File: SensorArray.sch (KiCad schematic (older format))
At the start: 13 parts

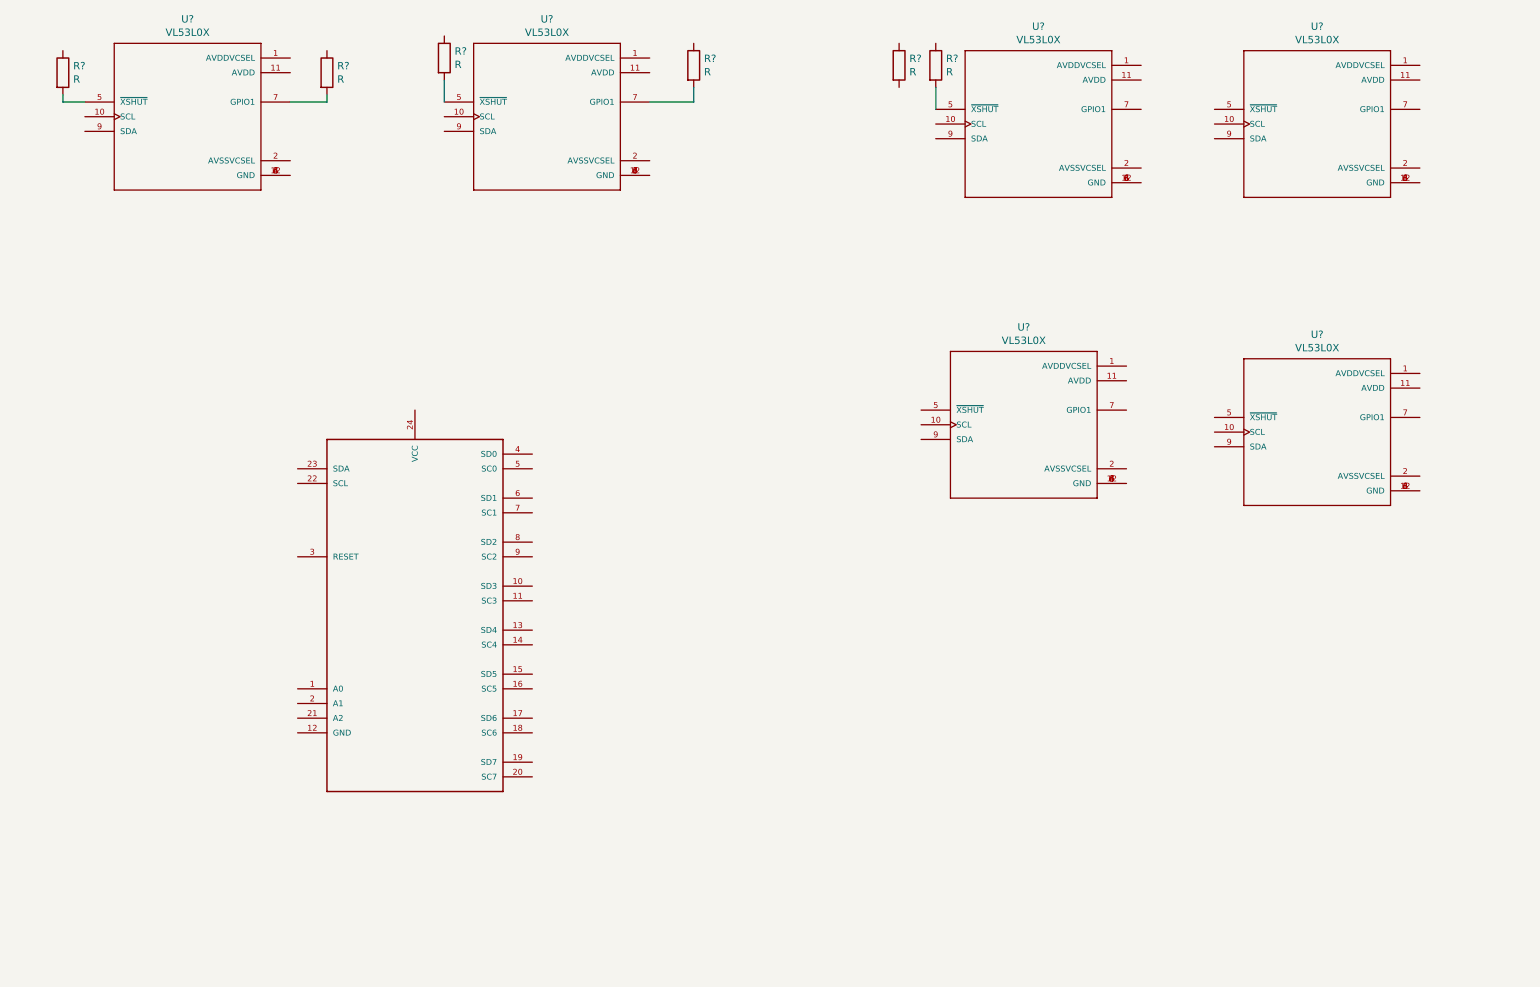
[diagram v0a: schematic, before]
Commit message: Week 6 Progress
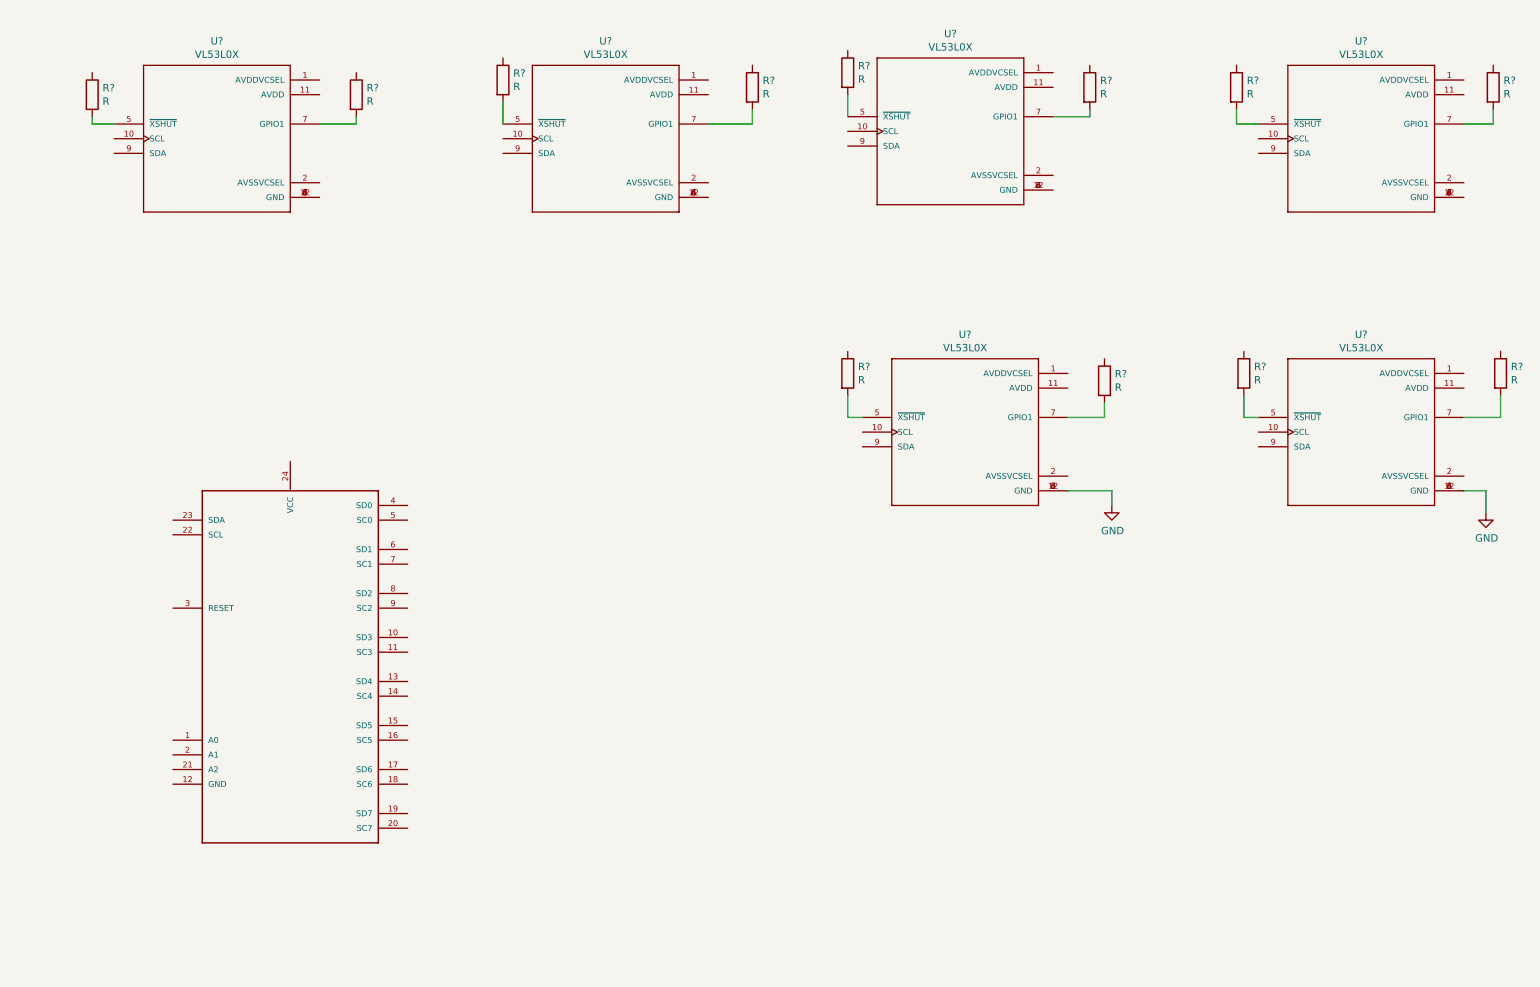
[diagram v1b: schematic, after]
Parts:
- added R? (x6): R, symbol device:R
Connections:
- net at U?.5 (~XSHUT~): now also R?.2 (x3)
- net at U?.7 (GPIO1): now also R?.2 (x4)
- net GND: now reaches U?.12 (GND), U?.3 (GND), U?.4 (GND), U?.6 (GND)
- net GND: now also U?.12 (GND), U?.3 (GND), U?.4 (GND), U?.6 (GND)
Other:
- moved on the sheet: R?, U?

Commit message: More Thinks finished week 7
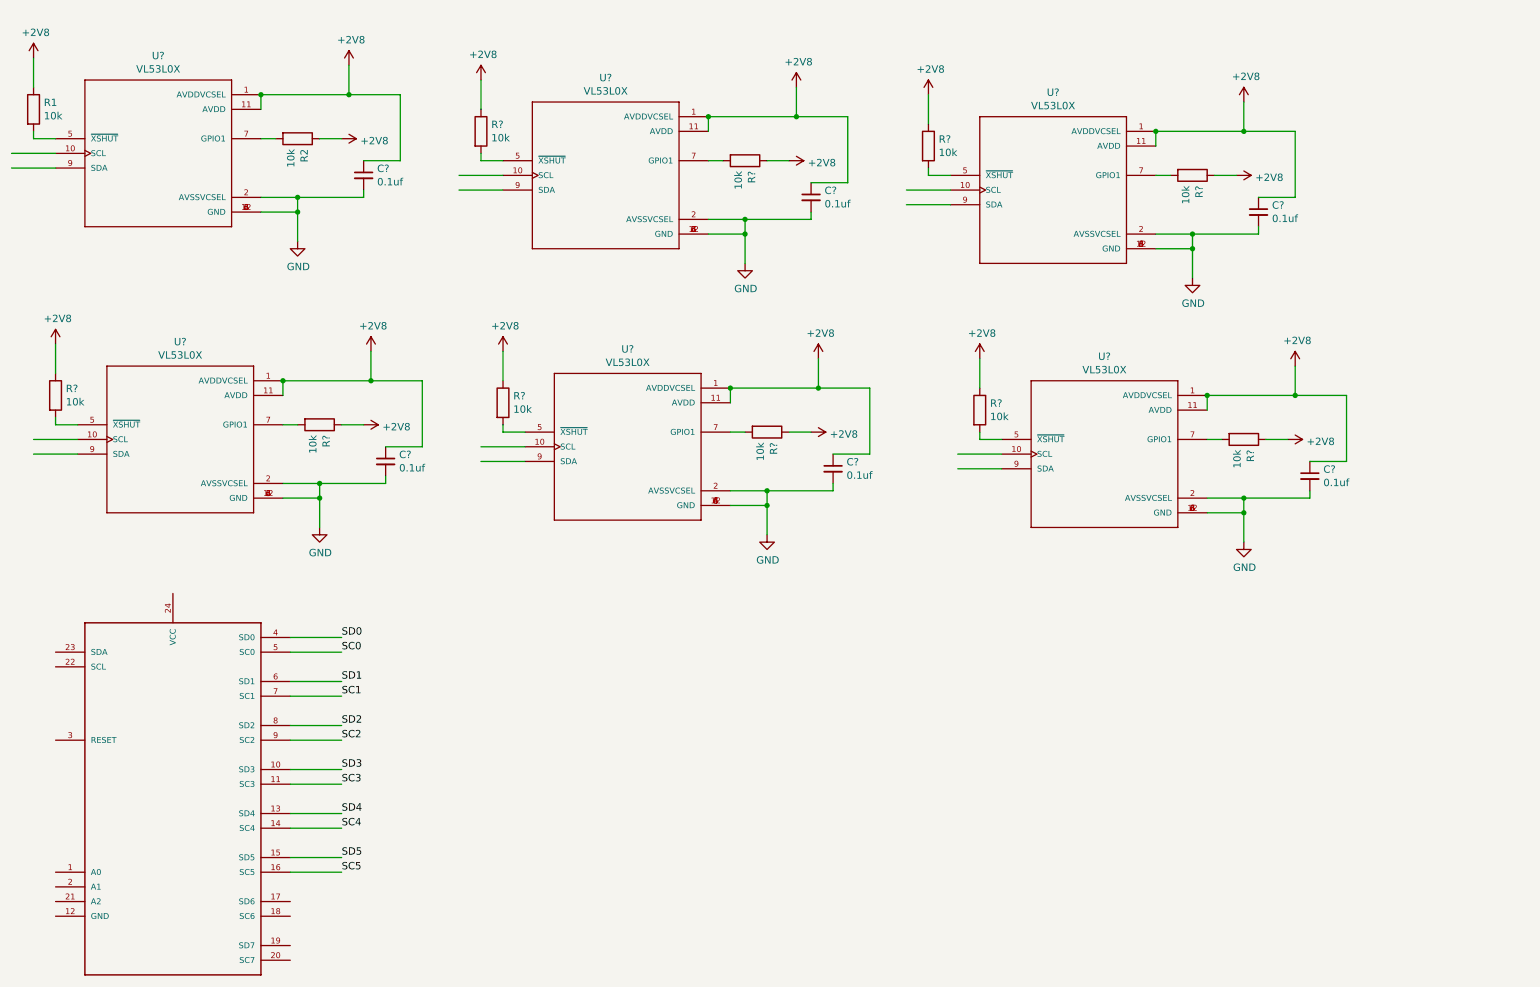
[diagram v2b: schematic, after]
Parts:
- removed R? (x10): R, symbol device:R
- removed U? (x5): VL53L0X, SENSOR_VL53L0X, symbol VL53L0X:VL53L0X
- added C? (x6): 0.1uf, symbol device:C_Small
- added R? (x10): 10k, symbol device:R
- added U? (x5): VL53L0X, SENSOR_VL53L0X, symbol VL53L0X:VL53L0X
- R1, R2: renamed from R?; value R -> 10k
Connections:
- net labels added: +2V8, SC0, SC1, SC2, SC3, SC4, SC5, SD0, SD1, SD2, SD3, SD4, SD5
- wire segments 26 -> 126
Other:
- moved on the sheet: R1, R2, U?
